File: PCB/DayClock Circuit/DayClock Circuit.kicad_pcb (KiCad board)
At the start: 2 copper layers, 100 x 100 mm, 42 parts, among them J1 molex 15-24-4441, J10 RGB_LED_Strip_Connector, J2 RJ45, J3 Conn_02x08_Odd_Even, J4 LED Matrix Power, J5 Lower Limit Switch, J6 Upper Limit Switch, J7 Stepper Motor, J8 RGB_LED_Strip_Connector, J9 RGB_LED_Strip_Connector, Q1 N-MOSFET, Q2 N-MOSFET, Q3 N-MOSFET, Q4 N-MOSFET, Q5 N-MOSFET, Q6 N-MOSFET, Q7 N-MOSFET, Q8 N-MOSFET, Q9 N-MOSFET, SW1 SW_DIP_x03, U1 Arduino_Mega2560_Shield, U2 DRV8825_module, U3 Tiny_RTC_DS1307

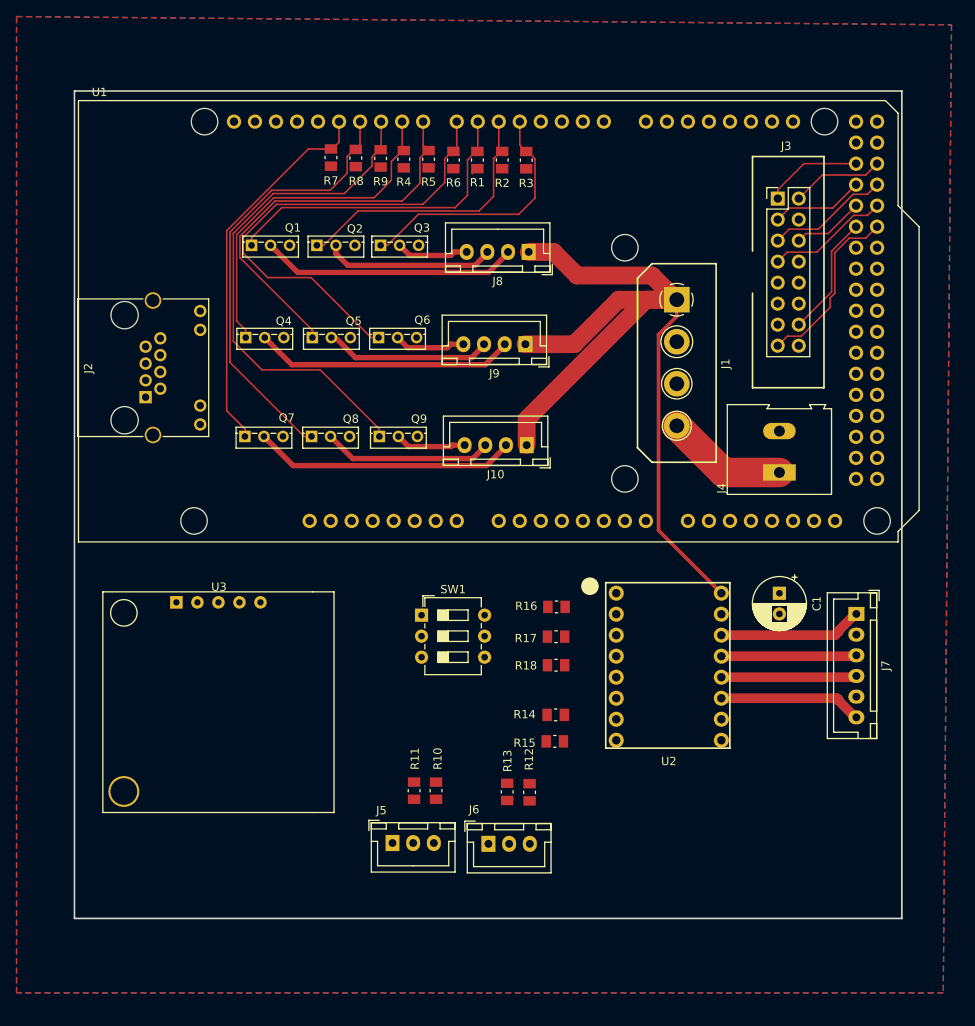
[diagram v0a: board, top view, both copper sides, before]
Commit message: Giant Day Cycle Clock Rev 1A sent to fab and components ordered
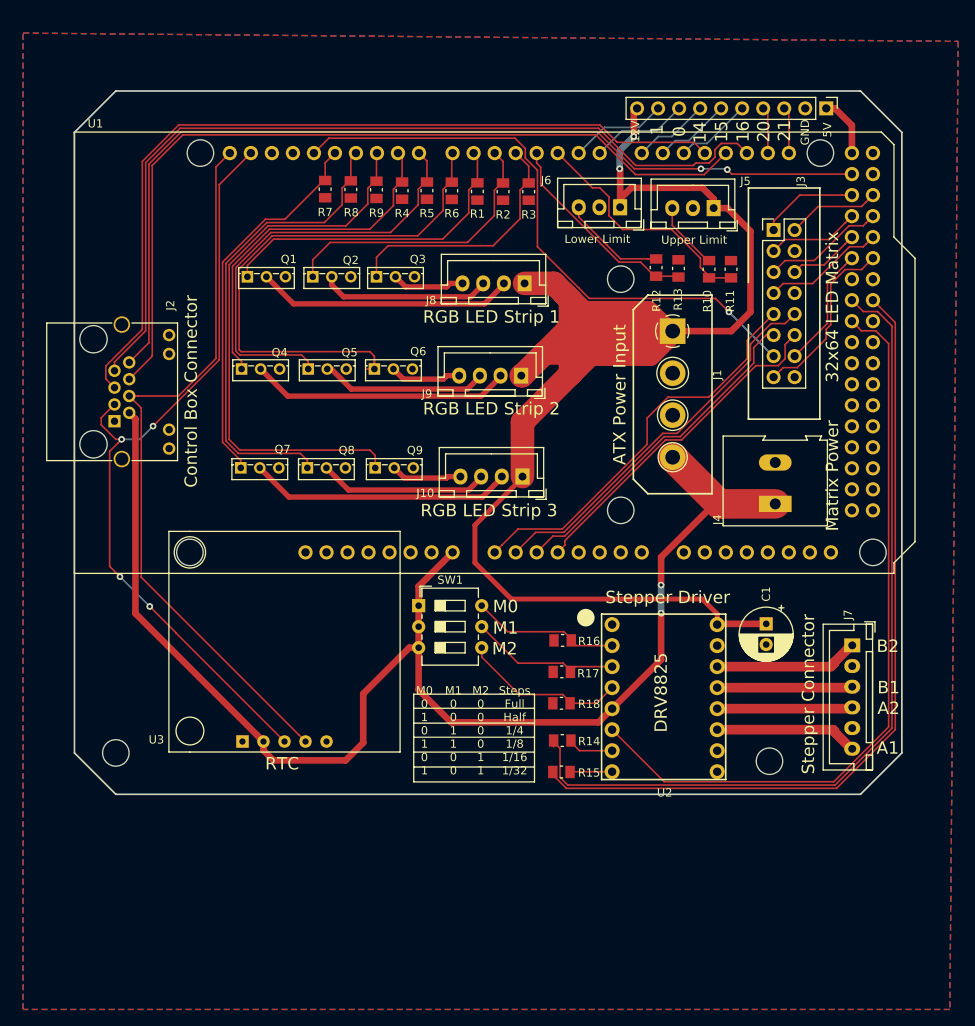
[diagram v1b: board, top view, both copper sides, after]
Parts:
- added J11: Breakout Pins, Connector_PinHeader_2.54mm:PinHeader_1x10_P2.54mm_Vertical, F.Cu at (105.9, 17.1)
- added REF**: MountingHole_3.2mm_M3, MountingHole:MountingHole_3.2mm_M3, F.Cu at (20.0, 95.0)
- added REF**: MountingHole_3.2mm_M3, MountingHole:MountingHole_3.2mm_M3, F.Cu at (99.0, 96.0)
- U3: footprint rich-footprints:TinyRTC-one-mounting-hole -> rich-footprints:TinyRTC-coin-side-up
- moved J5 86.0 mm to (92.2, 29.1), turned to 180 degrees
- moved J6 78.6 mm to (81.0, 29.1), turned to 180 degrees
- moved R11 73.7 mm to (94.3, 36.5), turned to 90 degrees
- moved R10 71.1 mm to (91.7, 36.5), turned to 270 degrees
- moved R13 66.6 mm to (88.0, 36.4), turned to 90 degrees
- moved R12 65.2 mm to (85.3, 36.3), turned to 270 degrees
- moved U3 40.2 mm to (55.6, 91.1), turned to 90 degrees
- moved J2 4.75 mm to (19.8, 54.9)
- moved R18 4.65 mm to (73.9, 89.0)
- moved R17 4.31 mm to (73.9, 85.2)
- moved R16 4.12 mm to (74.0, 81.4)
- moved C1 4.03 mm to (98.6, 79.4)
- moved R7 3.88 mm to (45.3, 26.9)
- moved R8 3.85 mm to (48.4, 26.9)
- moved U2 3.83 mm to (87.6, 89.7)
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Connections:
- U1 pad 5V3: (no net) -> /5V3
- U1 pad D0: (no net) -> /D0
- U1 pad D1: (no net) -> /D1
- U1 pad D14: (no net) -> /D14
- U1 pad D15: (no net) -> /D15
- U1 pad D16: (no net) -> /D16
- U1 pad D20: (no net) -> /D20
- U1 pad D21: (no net) -> /D21
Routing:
- net +5V: track 14.7 -> 166.1 mm, vias 0 -> 2
- net /D22: track 0.00 -> 113.7 mm, vias 0 -> 2
- net /D19: track 0.00 -> 105.1 mm
- net /D34: track 0.00 -> 103.0 mm
- net /D18: track 0.00 -> 100.9 mm
- net /D17: track 0.00 -> 100.8 mm
- net /D35: track 0.00 -> 98.4 mm
- net /SDA: track 0.00 -> 94.6 mm, vias 0 -> 4
- net /D36: track 0.00 -> 90.7 mm
- net /SCL: track 0.00 -> 88.5 mm
- net +12V: track 107.6 -> 191.0 mm, vias 0 -> 2
- net /D13: track 0.00 -> 73.3 mm, vias 0 -> 1
- net /A0: track 0.00 -> 48.8 mm
- net /A1: track 0.00 -> 46.8 mm
- net /A3: track 0.00 -> 40.8 mm
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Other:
- board size 100 x 100 mm -> 100 x 85 mm
- net class 12v: trace_width 1.1 -> 0.8
- net class 5v: trace_width 3.57 -> 0.8
- board text added: "0"
- board text added: "1"
- board text added: "12V"
- board text added: "14"
- board text added: "15"
- board text added: "16"
- board text added: "20"
- board text added: "21"
- board text added: "32x64 LED Matrix"
- board text added: "5V"
- board text added: "A1"
- board text added: "A2"
- board text added: "ATX Power Input"
- board text added: "B1"
- board text added: "B2"
- board text added: "Control Box Connector"
- board text added: "DRV8825"
- board text added: "GND"
- board text added: "Giant Day Cycle Clock Rev 1A"
- board text added: "Lower Limit"
- board text added: "M0"
- board text added: "M0 0 1 0 1 0 1"
- board text added: "M1"
- board text added: "M1 0 0 1 1 0 0"
- board text added: "M2"
- board text added: "M2 0 0 0 0 1 1"
- board text added: "Matrix Power"
- board text added: "RGB LED Strip 1"
- board text added: "RGB LED Strip 2"
- board text added: "RGB LED Strip 3"
- board text added: "RTC"
- board text added: "Rich Nelson 06/2018"
- board text added: "Stepper Connector"
- board text added: "Stepper Driver"
- board text added: "Steps Full Half 1/4 1/8 1/16 1/32"
- board text added: "Upper Limit"
